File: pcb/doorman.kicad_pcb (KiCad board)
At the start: 4 copper layers, 37.1 x 37.2 mm, 45 parts, among them J1 USB_C_Receptacle_USB2.0, J2 Terminal, J3 3V3 Test Pad, J4 Conn_02x07_Odd_Even, J6 BUS Test Pad, J7 BUS RX Test Pad, J8 TX Test Pad, J9 RX Test Pad, Q1 BC847BPN, Q2 BC817, SW1 Reset Button, SW2 Flash Button, U2 AP63203WU, U3 GAQY252G3S, U4 ESP32-S3-MINI-1

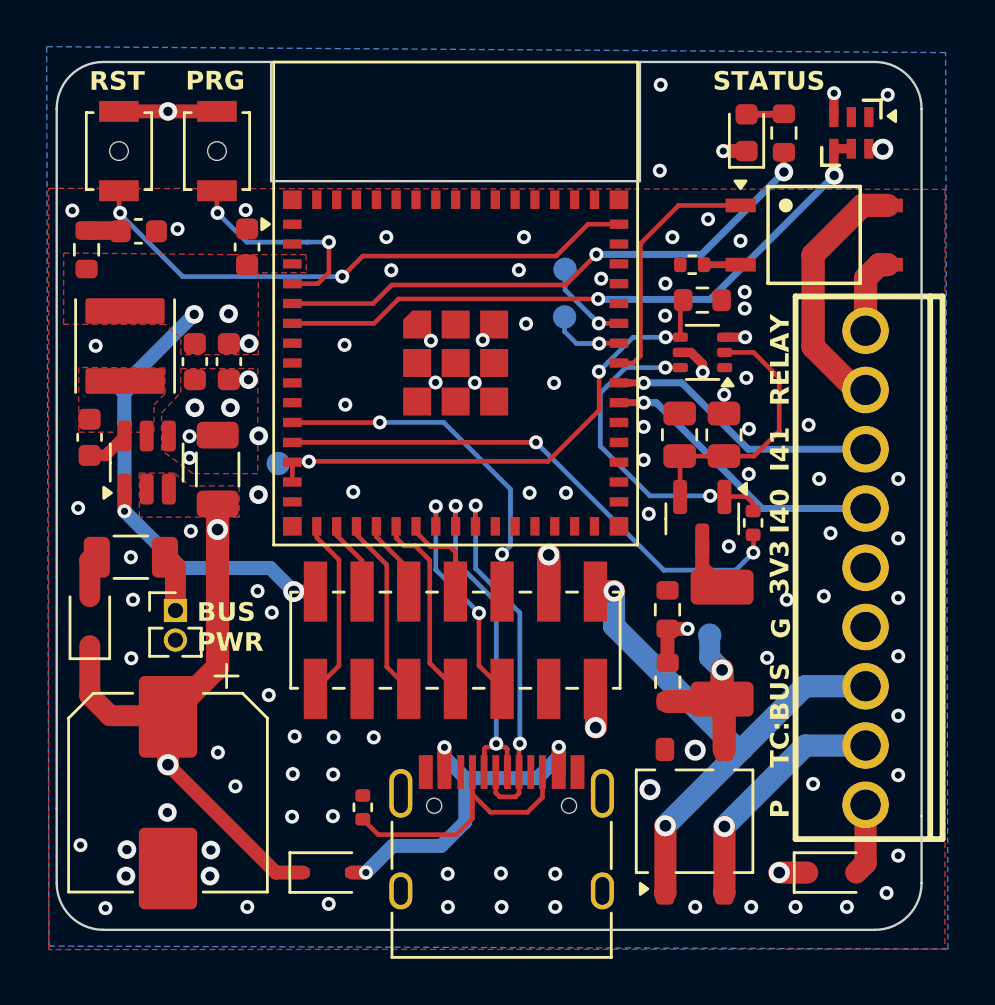
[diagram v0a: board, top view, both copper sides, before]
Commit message: WIP
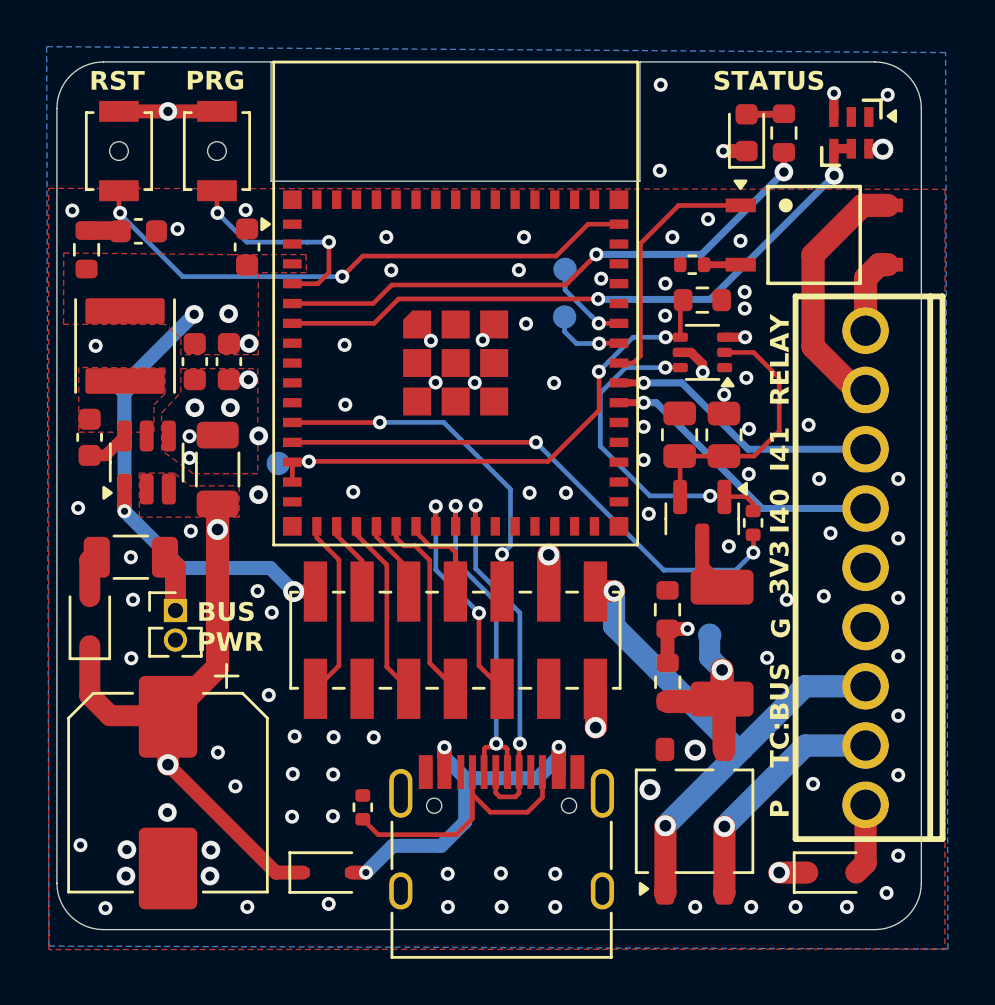
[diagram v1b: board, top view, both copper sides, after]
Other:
- board size 37.1 x 37.2 mm -> 37 x 37.2 mm
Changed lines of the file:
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@@
 		(layer "Dwgs.User")
 	)
-	(gr_line
-		(start 126.83033 108.68)
-		(end 126.83033 111.88)
+	(gr_arc
+		(start 161.9 76.68)
+		(mid 163.307144 77.262858)
+		(end 163.890002 78.670002)
 		(stroke
-			(width 0.1)
+			(width 0.05)
 			(type default)
 		)
@@
 	)
 	(gr_line
-		(start 163.9 109)
-		(end 163.9 111.88)
+		(start 136.02 76.68)
+		(end 136.02 81.79)
 		(stroke
-			(width 0.1)
-			(type default)
-		)
-		(layer "Edge.Cuts")
-	)
-	(gr_arc
-		(start 163.9 111.88)
-		(mid 163.314215 113.294224)
-		(end 161.9 113.88)
-		(stroke
-			(width 0.1)
-			(type default)
-		)
-		(layer "Edge.Cuts")
-	)
-	(gr_line
-		(start 126.83033 108.68)
-		(end 126.83033 78.68)
-		(stroke
-			(width 0.1)
+			(width 0.05)
 			(type default)
 		)
@@
 		(end 151.83 81.79)
 		(stroke
-			(width 0.1)
+			(width 0.05)
 			(type default)
 		)
@@
 		(end 136.02 81.79)
 		(stroke
-			(width 0.1)
+			(width 0.05)
+			(type default)
+		)
+		(layer "Edge.Cuts")
+	)
+	(gr_line
+		(start 161.9 113.870002)
+		(end 128.83033 113.870002)
+		(stroke
+			(width 0.05)
+			(type default)
+		)
+		(layer "Edge.Cuts")
+	)
+	(gr_line
+		(start 163.890002 78.670002)
+		(end 163.890002 111.88)
+		(stroke
+			(width 0.05)
 			(type default)
 		)
@@
 	)
 	(gr_arc
-		(start 126.83033 78.68)
-		(mid 127.416116 77.265786)
+		(start 126.840328 78.670002)
+		(mid 127.423186 77.262858)
 		(end 128.83033 76.68)
 		(stroke
-			(width 0.1)
+			(width 0.05)
 			(type default)
 		)
@@
 	)
 	(gr_line
-		(start 161.9 113.88)
-		(end 128.83033 113.88)
+		(start 126.840328 78.670002)
+		(end 126.840328 111.88)
 		(stroke
-			(width 0.1)
-			(type default)
-		)
-		(layer "Edge.Cuts")
-	)
-	(gr_line
-		(start 163.899999 78.7)
-		(end 163.9 109)
-		(stroke
-			(width 0.1)
+			(width 0.05)
 			(type default)
 		)
@@
 	)
 	(gr_arc
-		(start 128.83033 113.88)
-		(mid 127.416116 113.294214)
-		(end 126.83033 111.88)
+		(start 128.83033 113.870002)
+		(mid 127.423186 113.287144)
+		(end 126.840328 111.88)
 		(stroke
-			(width 0.1)
-			(type default)
-		)
-		(layer "Edge.Cuts")
-	)
-	(gr_arc
-		(start 161.9 76.679871)
-		(mid 163.321339 77.272795)
-		(end 163.899999 78.7)
-		(stroke
-			(width 0.1)
+			(width 0.05)
 			(type default)
 		)
@@
 		(end 136.02 76.68)
 		(stroke
-			(width 0.1)
-			(type default)
-		)
-		(layer "Edge.Cuts")
-	)
-	(gr_line
-		(start 136.02 81.79)
-		(end 136.02 76.68)
-		(stroke
-			(width 0.1)
+			(width 0.05)
 			(type default)
 		)
@@
 		(end 161.9 76.68)
 		(stroke
-			(width 0.1)
+			(width 0.05)
 			(type default)
 		)
+		(layer "Edge.Cuts")
+	)
+	(gr_arc
+		(start 163.890002 111.88)
+		(mid 163.307144 113.287144)
+		(end 161.9 113.870002)
+		(stroke
+			(width 0.05)
+			(type default)
+		)
